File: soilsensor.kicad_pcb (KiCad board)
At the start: 2 copper layers, 23 x 113 mm, 32 parts, among them J1 CONN_01X07, J2 BATT_CONN, P1 USB_OTG, Q1 Q_NMOS_GSD, Q2 Q_PMOS_GSD, Q3 Q_PMOS_GSD, U1 DS18B20U, U2 RFD77101, U3 MCP73811T, U4 AP2204K-3.0, U5 TLC555

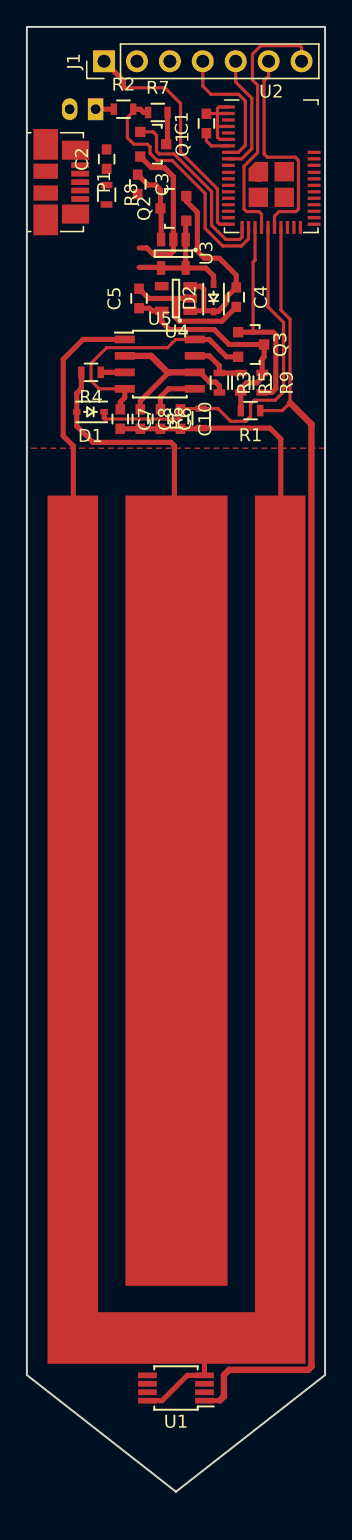
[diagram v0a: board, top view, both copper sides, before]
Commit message: update pcb
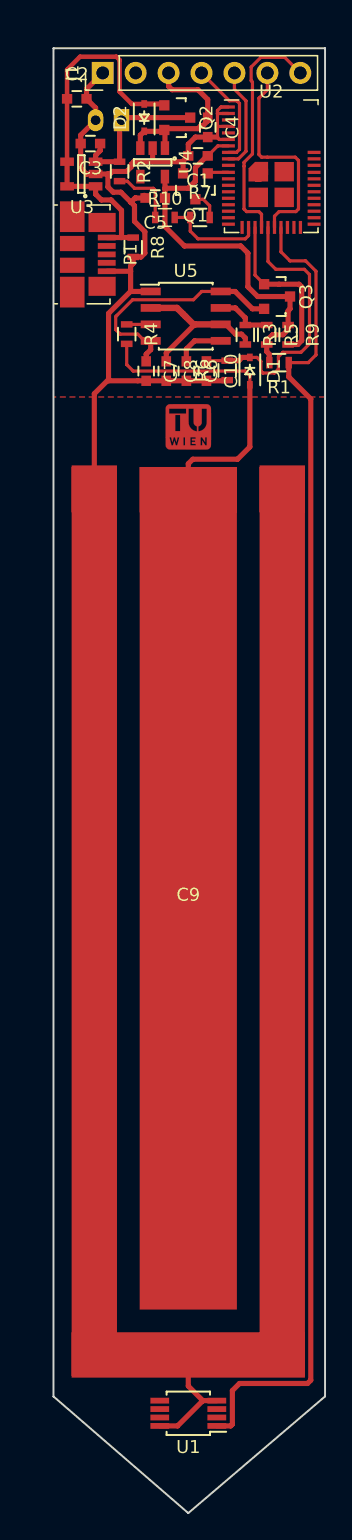
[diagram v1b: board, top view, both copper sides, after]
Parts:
- added G***: LOGO, LOGO, F.Cu at (105.5, 72.8)
- added R10: 1.8k, Resistors_SMD:R_0603, F.Cu at (103.7, 56.7)
- C9: footprint SoilMeasuringBoard:coil_sensor -> SoilMeasuringBoard:C_Sensor
- R2: value 3.3k -> 1.5k
- moved D2 14.9 mm to (102.0, 49.0)
- moved C4 13.3 mm to (107.0, 49.8)
- moved D1 12.7 mm to (110.2, 68.5), turned to 270 degrees
- moved U4 10.7 mm to (102.7, 52.5), turned to 270 degrees
- moved U3 9.39 mm to (97.2, 53.4), turned to 180 degrees
- moved R7 8.73 mm to (106.3, 56.7)
- moved C5 7.85 mm to (102.9, 55.2), turned to 180 degrees
- moved Q2 7.01 mm to (104.6, 49.0), turned to 270 degrees
- moved P1 5.94 mm to (96.5, 59.5)
- moved C2 5.19 mm to (96.8, 47.5), turned to 0 degrees
- moved C3 4.82 mm to (97.9, 51.0), turned to 180 degrees
- moved R2 4.81 mm to (100.2, 53.1), turned to 270 degrees
- moved Q1 4.60 mm to (106.0, 54.3), turned to 180 degrees
- moved R8 4.54 mm to (101.2, 59.0)
- moved R1 4.30 mm to (112.5, 67.9)
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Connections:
- net /CapacitiveSoilSensor/SensorOut renamed /SS_OUT
- net /CapacitiveSoilSensor/~EN renamed /~SS_EN
- J1 pad 2: (no net) -> Net-(J1-Pad2)
- P1 pad 2: (no net) -> Net-(P1-Pad2)
- P1 pad 3: (no net) -> Net-(P1-Pad3)
- P1 pad 4: (no net) -> Net-(P1-Pad4)
- Q1 pad 1: /PowerMgmt/BATT_V_EN -> /V_BATT_EN
- R2 pad 2: /PowerMgmt/BATT_V -> Net-(R10-Pad1)
- R7 pad 1: /PowerMgmt/BATT_V -> /V_BATT
- U1 pad 2: (no net) -> Net-(U1-Pad2)
- U1 pad 3: (no net) -> Net-(U1-Pad3)
- U1 pad 5: (no net) -> Net-(U1-Pad5)
- U1 pad 6: (no net) -> Net-(U1-Pad6)
- U1 pad 7: (no net) -> Net-(U1-Pad7)
- U2 pad 10: (no net) -> Net-(U2-Pad10)
- U2 pad 11: (no net) -> /V_BATT_EN
- U2 pad 12: (no net) -> Net-(U2-Pad12)
- U2 pad 13: (no net) -> Net-(U2-Pad13)
- U2 pad 14: (no net) -> Net-(U2-Pad14)
- U2 pad 15: (no net) -> Net-(U2-Pad15)
- U2 pad 16: (no net) -> Net-(U2-Pad16)
- U2 pad 17: (no net) -> Net-(U2-Pad17)
- U2 pad 18: (no net) -> Net-(U2-Pad18)
- U2 pad 20: /PowerMgmt/BATT_V_EN -> Net-(U2-Pad20)
- U2 pad 21: /PowerMgmt/BATT_V -> /V_BATT
- U2 pad 27: (no net) -> Net-(U2-Pad27)
- U2 pad 28: (no net) -> Net-(U2-Pad28)
- U2 pad 29: (no net) -> Net-(U2-Pad29)
- U2 pad 3: (no net) -> Net-(U2-Pad3)
- U2 pad 31: (no net) -> Net-(U2-Pad31)
- U2 pad 32: (no net) -> Net-(U2-Pad32)
- U2 pad 33: (no net) -> Net-(U2-Pad33)
- U2 pad 34: (no net) -> Net-(U2-Pad34)
- U2 pad 35: (no net) -> Net-(U2-Pad35)
- U2 pad 36: (no net) -> Net-(U2-Pad36)
- U2 pad 37: (no net) -> Net-(U2-Pad37)
- U2 pad 38: (no net) -> Net-(U2-Pad38)
- U2 pad 39: (no net) -> Net-(U2-Pad39)
- U2 pad 40: (no net) -> Net-(U2-Pad40)
- U2 pad 41: (no net) -> Net-(U2-Pad41)
- U2 pad 5: (no net) -> Net-(U2-Pad5)
- U4 pad 4: (no net) -> Net-(U4-Pad4)
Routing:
- net GND: track 162.1 -> 113.5 mm
- net Net-(C9-Pad1): track 18.2 -> 55.0 mm
- net /PowerMgmt/BATT_V: track 19.4 -> 0.00 mm
- net Net-(C2-Pad1): track 10.3 -> 29.4 mm
- net /PowerMgmt/BATT_V_EN: track 14.4 -> 0.00 mm
- net VDD: track 20.1 -> 30.6 mm
- net /SS_OUT: track 30.1 -> 22.1 mm
- net /V_BATT: track 0.00 -> 7.73 mm
- net Net-(R10-Pad1): track 0.00 -> 5.34 mm
- net +BATT: track 7.50 -> 12.0 mm
- net /~SS_EN: track 16.4 -> 13.0 mm
- net VBUS: track 16.7 -> 14.2 mm
- net /SWDIO/RESET: track 10.6 -> 8.40 mm
- net /GPIO1: track 20.3 -> 18.4 mm
- net Net-(R1-Pad1): track 101.7 -> 103.4 mm
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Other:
- board size 23 x 113 mm -> 21 x 113 mm
